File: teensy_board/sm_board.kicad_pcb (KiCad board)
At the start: 2 copper layers, 70.5 x 42.5 mm, 45 parts, among them J0 CONN_01X03, J1 CONN_01X03, J10 CONN_01X04, J11 CONN_01X02, J12 CONN_02X04, J2 CONN_01X03, J3 CONN_01X03, J4 CONN_01X03, J5 CONN_01X03, J6 CONN_01X03, J7 CONN_01X02, J8 CONN_01X02, J9 CONN_01X04, U1 Teensy3.6, U2 drv8833, U3 tps82130

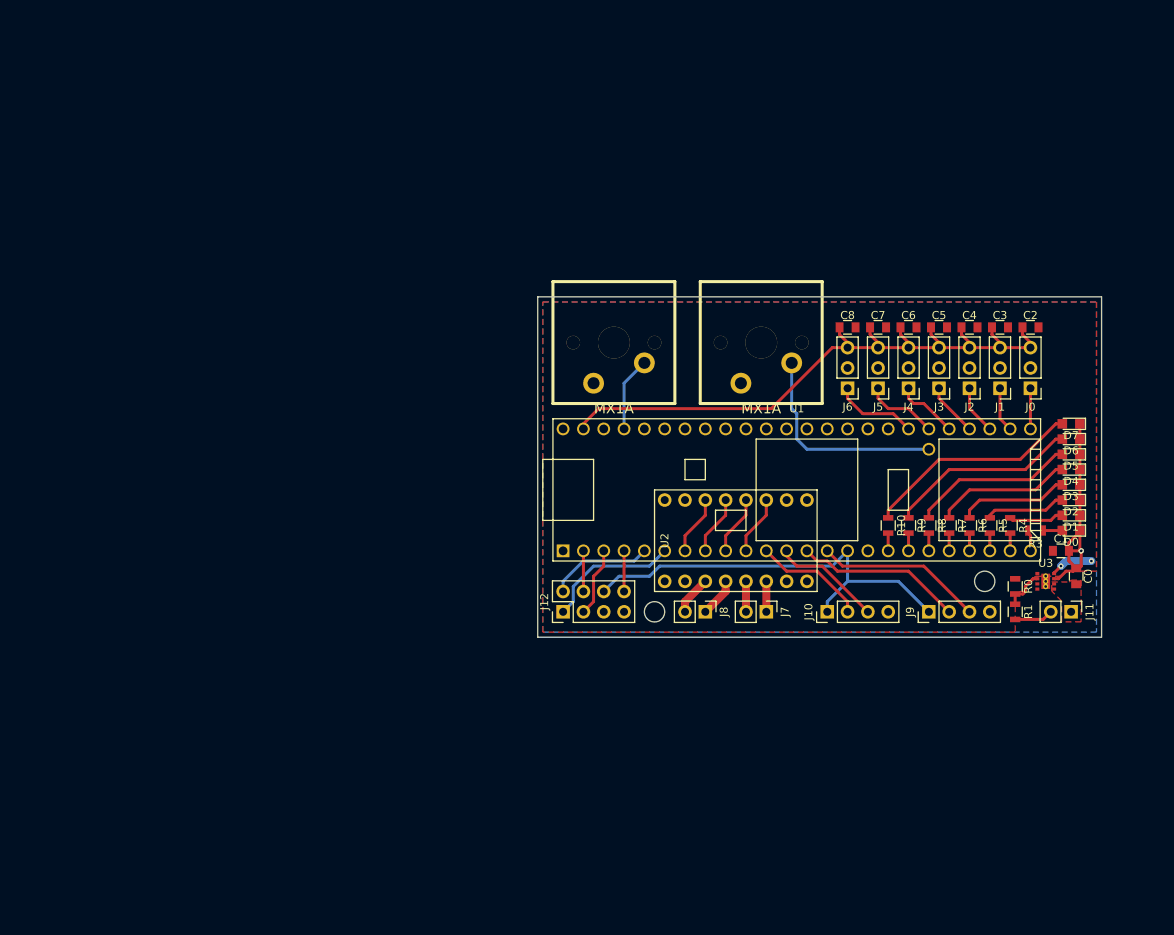
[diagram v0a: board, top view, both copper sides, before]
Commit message: I think im done the schematic for tonight
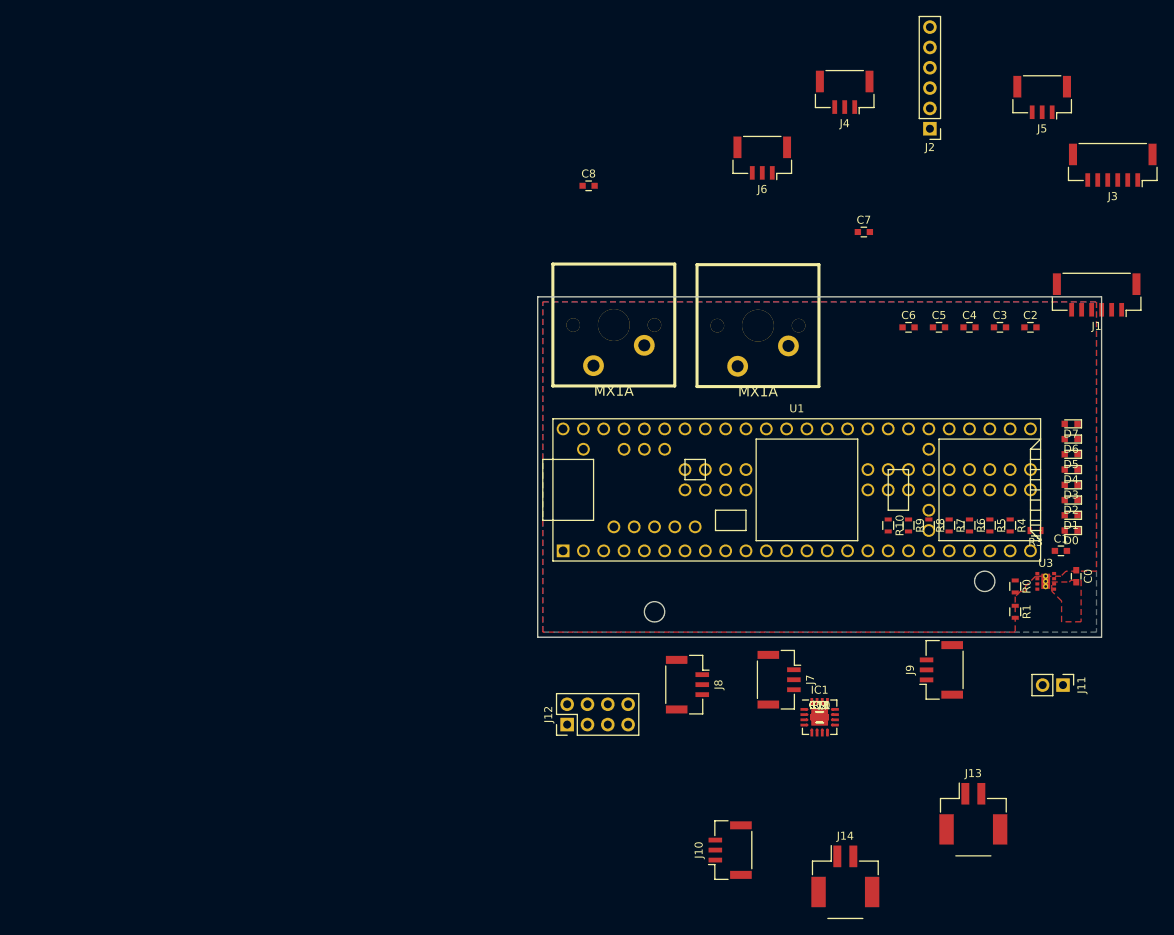
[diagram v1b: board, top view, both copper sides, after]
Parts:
- removed J0: CONN_01X03, Pin_Headers:Pin_Header_Straight_1x03_Pitch2.54mm
- removed U2: drv8833, drv8833:drv8833
- added C10: 0.01uC, Capacitors_SMD:C_0603, F.Cu at (126.0, 119.9)
- added C11: 10uC, Capacitors_SMD:C_0603, F.Cu at (126.0, 119.9)
- added C9: 2.2uC, Capacitors_SMD:C_0603, F.Cu at (126.0, 119.9)
- added IC1: DRV8833RTYT, Housings_DFN_QFN:WQFN-16-1EP_4x4mm_Pitch0.65mm, F.Cu at (126.0, 119.9)
- added J13: Conn_01x02, Connector_Molex:Molex_CLIK-Mate_502494-0270_1x02_P2.00mm_Horizontal, F.Cu at (145.3, 131.9)
- added J14: Conn_01x02, Connector_Molex:Molex_CLIK-Mate_502494-0270_1x02_P2.00mm_Horizontal, F.Cu at (129.3, 139.8)
- added R11, R2: R, Resistors_SMD:R_0603, F.Cu at (126.0, 119.9)
- C0, C1, C2, C3, C4, C5, C6, C7, C8: footprint Capacitors_SMD:C_0805 -> Capacitors_SMD:C_0603
- D0, D1, D2, D3, D4, D5, D6, D7: footprint LEDs:LED_0805 -> LEDs:LED_0603
- J1, J3: value CONN_01X03 -> Conn_01x06; footprint Pin_Headers:Pin_Header_Straight_1x03_Pitch2.54mm -> Connector_Molex:Molex_CLIK-Mate_502386-0670_1x06_P1.25mm_Horizontal
- J10, J9: value CONN_01X04 -> Conn_01x03; footprint Pin_Headers:Pin_Header_Straight_1x04_Pitch2.54mm -> Connector_Molex:Molex_CLIK-Mate_502386-0370_1x03_P1.25mm_Horizontal
- J2: value CONN_01X03 -> Conn_01x06; footprint Pin_Headers:Pin_Header_Straight_1x03_Pitch2.54mm -> Pin_Headers:Pin_Header_Straight_1x06_Pitch2.54mm
- J4, J5, J6: value CONN_01X03 -> Conn_01x03; footprint Pin_Headers:Pin_Header_Straight_1x03_Pitch2.54mm -> Connector_Molex:Molex_CLIK-Mate_502386-0370_1x03_P1.25mm_Horizontal
- J7, J8: value CONN_01X02 -> Conn_01x03; footprint Pin_Headers:Pin_Header_Straight_1x02_Pitch2.54mm -> Connector_Molex:Molex_CLIK-Mate_502386-0370_1x03_P1.25mm_Horizontal
- R0, R1, R10, R3, R4, R5, R6, R7, R8, R9: footprint Resistors_SMD:R_0805 -> Resistors_SMD:R_0603
- U1: footprint Teensy:Teensy35_36_reset -> Teensy:Teensy35_36
- moved J5 41.7 mm to (153.9, 42.4)
- moved J4 37.9 mm to (129.2, 41.7)
- moved C8 36.9 mm to (97.2, 53.4)
- moved J3 35.3 mm to (162.7, 50.9)
- moved J2 32.8 mm to (139.8, 46.3)
- moved J10 32.2 mm to (114.9, 136.5)
- moved J6 30.7 mm to (118.9, 50.0)
- moved J1 16.8 mm to (160.7, 67.1)
- moved J12 14.1 mm to (94.5, 120.8)
- moved C7 12.0 mm to (131.6, 59.2)
- moved J8 9.37 mm to (109.5, 115.8)
- moved J11 9.22 mm to (156.5, 115.8)
- moved J7 8.64 mm to (121.0, 115.2)
- moved J9 7.43 mm to (141.3, 113.9)
- moved S1 2.19 mm to (100.3, 70.8)
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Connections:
- J1 pad 1: dist_a_1 -> MOSI
- J1 pad 2: +5V -> MISO
- J1 pad 3: GNDA -> SCK
- J10 pad 1: +3V3 -> dist_a_6
- J10 pad 2: enc_a1 -> +5V
- J10 pad 3: enc_a2 -> GNDA
- J2 pad 1: dist_a_2 -> Net-(J2-Pad1)
- J2 pad 2: +5V -> tx_imu
- J2 pad 3: GNDA -> rx_imu
- J3 pad 1: dist_a_3 -> MOSI
- J3 pad 2: +5V -> MISO
- J3 pad 3: GNDA -> SCK
- J4 pad 1: dist_a_4 -> dist_a_0
- J5 pad 1: dist_a_5 -> dist_a_1
- J6 pad 1: dist_a_6 -> dist_a_2
- J7 pad 1: Net-(J7-Pad1) -> dist_a_3
- J7 pad 2: Net-(J7-Pad2) -> +5V
- J8 pad 1: Net-(J8-Pad1) -> dist_a_4
- J8 pad 2: Net-(J8-Pad2) -> +5V
- J9 pad 1: +3V3 -> dist_a_5
- J9 pad 2: enc_b1 -> +5V
- J9 pad 3: enc_b2 -> GNDA
- U1 pad 11: enc_a1 -> MOSI
- U1 pad 12: enc_a2 -> MISO
- U1 pad 13: enc_b1 -> CS0
- U1 pad 14: enc_b2 -> CS1
- U1 pad 40: Net-(U1-Pad40) -> SCK
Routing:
- net GNDA: track 81.1 -> 0.00 mm
- net +3V3: track 53.0 -> 0.00 mm
- net GND: track 33.9 -> 0.00 mm, vias 1 -> 0
- net Net-(D7-Pad2): track 27.2 -> 0.00 mm
- net sw_0: track 26.8 -> 0.00 mm
- net Net-(D6-Pad2): track 23.9 -> 0.00 mm
- net enc_b1: track 20.9 -> 0.00 mm
- net enc_b2: track 20.9 -> 0.00 mm
- net Net-(D5-Pad2): track 20.5 -> 0.00 mm
- net Net-(D4-Pad2): track 17.2 -> 0.00 mm
- net sda_imu: track 17.0 -> 0.00 mm
- net enc_a1: track 14.7 -> 0.00 mm
- net Net-(D3-Pad2): track 13.9 -> 0.00 mm
- net enc_a2: track 13.7 -> 0.00 mm
- net scl_imu: track 13.0 -> 0.00 mm
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
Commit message: pre-meeting board layout
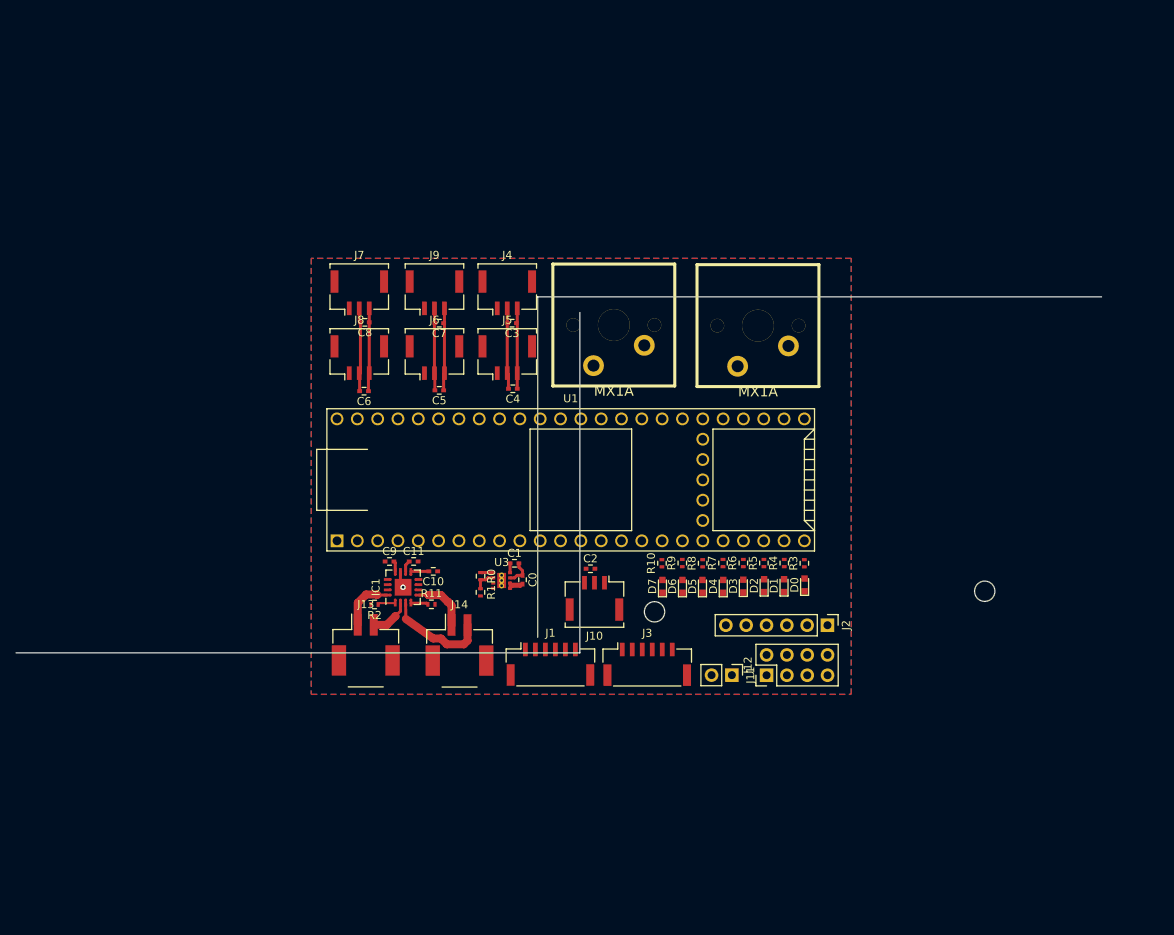
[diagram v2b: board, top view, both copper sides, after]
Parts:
- C0, C1, C10, C11, C2, C3, C4, C5, C6, C7, C8, C9: footprint Capacitors_SMD:C_0603 -> Capacitors_SMD:C_0402
- J10, J4, J5, J6, J7, J8, J9: footprint Connector_Molex:Molex_CLIK-Mate_502386-0370_1x03_P1.25mm_Horizontal -> Connector_Molex:Molex_CLIK-Mate_502382-0370_1x03_P1.25mm_Vertical
- R0, R1, R10, R11, R2, R3, R4, R5, R6, R7, R8, R9: footprint Resistors_SMD:R_0603 -> Resistors_SMD:R_0402
- U1: footprint Teensy:Teensy35_36 -> Teensy2:Teensy35_36_custom
- moved J3 85.3 mm to (104.5, 113.2), turned to 0 degrees
- moved J1 82.4 mm to (92.4, 113.2), turned to 0 degrees
- moved J9 79.0 mm to (77.9, 66.8), turned to 0 degrees
- moved J13 78.8 mm to (69.3, 110.8)
- moved J5 74.3 mm to (87.0, 74.9), turned to 0 degrees
- moved J7 71.4 mm to (68.5, 66.8), turned to 0 degrees
- moved C0 69.2 mm to (88.9, 102.7)
- moved C6 68.5 mm to (69.1, 79.1), turned to 180 degrees
- moved C1 68.3 mm to (87.9, 100.6)
- moved U3 68.0 mm to (86.3, 102.8)
- moved R1 66.9 mm to (83.6, 104.2)
- moved R0 66.8 mm to (83.7, 102.2)
- moved J2 63.4 mm to (127.0, 108.4), turned to 270 degrees
- moved C5 63.0 mm to (78.5, 79.0), turned to 180 degrees
- moved C2 62.7 mm to (97.4, 101.3)
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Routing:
- net +5V: track 0.00 -> 33.6 mm
- net GNDA: track 0.00 -> 30.7 mm
- net m2b: track 0.00 -> 12.9 mm
- net m2a: track 0.00 -> 7.05 mm
- net m1a: track 0.00 -> 6.88 mm
- net GND: track 0.00 -> 5.51 mm, vias 0 -> 1
- net m1b: track 0.00 -> 5.05 mm
- net +BATT: track 0.00 -> 4.04 mm
- net Net-(R0-Pad2): track 0.00 -> 2.81 mm
- net Net-(C10-Pad2): track 0.00 -> 2.25 mm
- net Net-(IC1-Pad1): track 0.00 -> 2.21 mm
- net Net-(IC1-Pad4): track 0.00 -> 2.18 mm
- net Net-(C11-Pad1): track 0.00 -> 1.42 mm
- net Net-(C9-Pad2): track 0.00 -> 1.30 mm
- removed copper zone on F.Cu, net +BATT
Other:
- board size 70.5 x 42.5 mm -> 135.7 x 44.5 mm

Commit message: I think this is done
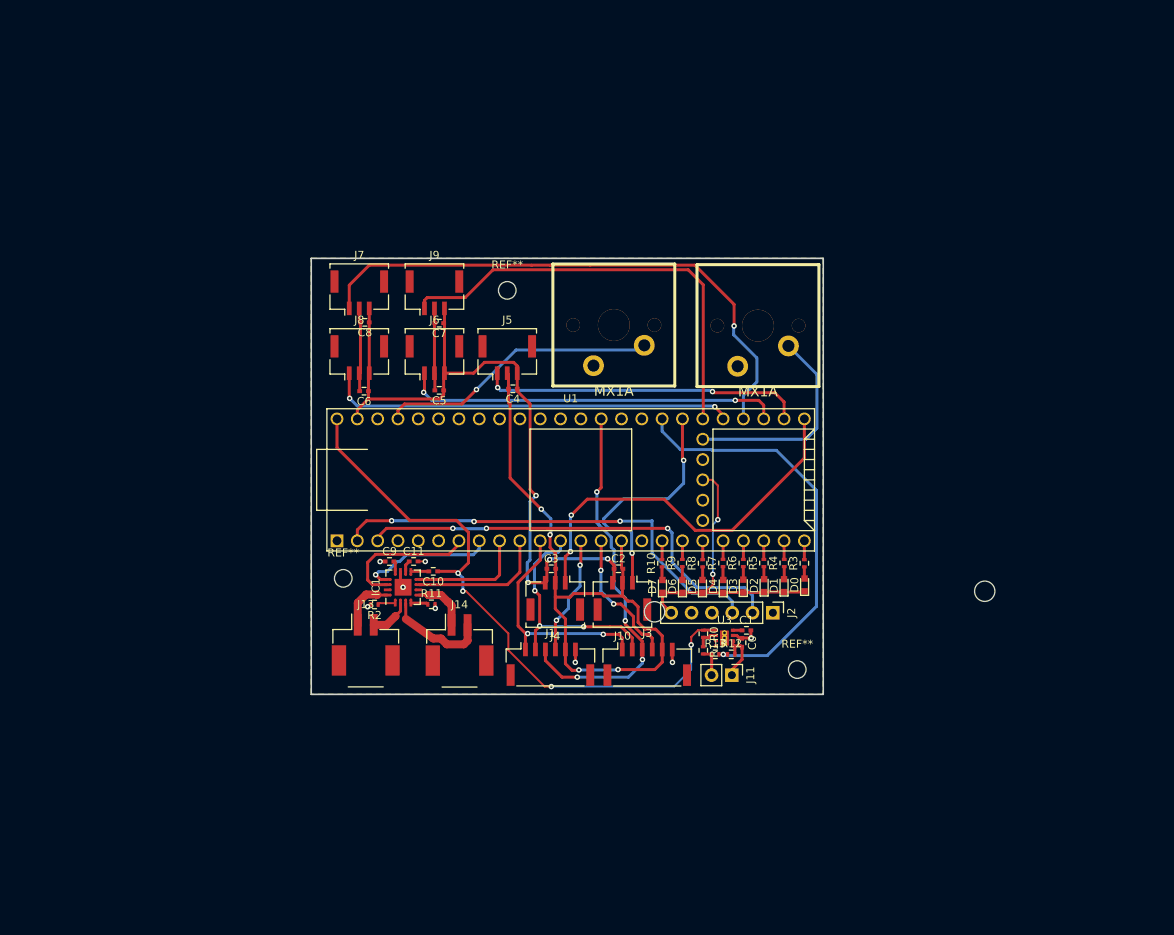
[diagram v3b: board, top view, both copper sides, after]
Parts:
- removed J12: CONN_02X04, Pin_Headers:Pin_Header_Straight_2x04_Pitch2.54mm
- added R12: R, Resistors_SMD:R_0402, F.Cu at (115.0, 112.0)
- added R13: R, Resistors_SMD:R_0402, F.Cu at (113.0, 112.0)
- added REF**: MountingHole_2.2mm_M2, Mounting_Holes:MountingHole_2.2mm_M2, F.Cu at (87.0, 66.5)
- added REF**: MountingHole_2.2mm_M2, Mounting_Holes:MountingHole_2.2mm_M2, F.Cu at (66.5, 102.5)
- added REF**: MountingHole_2.2mm_M2, Mounting_Holes:MountingHole_2.2mm_M2, F.Cu at (123.2, 113.9)
- moved J4 38.7 mm to (93.0, 105.0), turned to 180 degrees
- moved C3 31.1 mm to (92.5, 101.3), turned to 0 degrees
- moved C1 30.2 mm to (116.9, 109.0)
- moved R1 28.8 mm to (111.5, 111.5)
- moved R0 28.8 mm to (111.5, 109.4)
- moved U3 28.8 mm to (114.1, 110.0)
- moved C0 28.5 mm to (116.3, 110.5)
- moved J2 7.00 mm to (120.2, 106.8)
- moved C2 3.50 mm to (100.9, 101.3)
- moved J10 3.50 mm to (101.4, 105.0)
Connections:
- C2 pad 2: +5V -> +3V3
- C3 pad 2: +5V -> +3V3
- C4 pad 2: +5V -> +3V3
- C5 pad 2: +5V -> +3V3
- C6 pad 2: +5V -> +3V3
- C7 pad 2: +5V -> +3V3
- C8 pad 2: +5V -> +3V3
- J10 pad 2: +5V -> +3V3
- J4 pad 2: +5V -> +3V3
- J5 pad 2: +5V -> +3V3
- J6 pad 2: +5V -> +3V3
- J7 pad 2: +5V -> +3V3
- J8 pad 2: +5V -> +3V3
- J9 pad 2: +5V -> +3V3
- U1 pad 37: Net-(U1-Pad37) -> BattCheck
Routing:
- net +3V3: track 0.00 -> 100.2 mm, vias 0 -> 4
- net dist_a_3: track 0.00 -> 70.3 mm, vias 0 -> 1
- net GNDA: track 30.7 -> 89.3 mm, vias 0 -> 4
- net rx_imu: track 0.00 -> 56.8 mm, vias 0 -> 3
- net tx_imu: track 0.00 -> 55.6 mm, vias 0 -> 3
- net dist_a_5: track 0.00 -> 55.0 mm
- net BattCheck: track 0.00 -> 53.8 mm, vias 0 -> 1
- net GND: track 5.51 -> 57.8 mm, vias 1 -> 10
- net dist_a_4: track 0.00 -> 51.2 mm, vias 0 -> 2
- net dist_a_0: track 0.00 -> 49.0 mm, vias 0 -> 2
- net SCK: track 0.00 -> 48.2 mm, vias 0 -> 4
- net dist_a_2: track 0.00 -> 47.3 mm, vias 0 -> 2
- net +5V: track 33.6 -> 79.5 mm, vias 0 -> 4
- net dist_a_1: track 0.00 -> 40.5 mm, vias 0 -> 2
- net sw_1: track 0.00 -> 35.2 mm, vias 0 -> 1
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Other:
- board size 135.7 x 44.5 mm -> 85.5 x 54.5 mm
